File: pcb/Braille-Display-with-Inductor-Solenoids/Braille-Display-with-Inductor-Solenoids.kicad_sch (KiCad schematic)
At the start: 30 parts, among them J1 Screw_Terminal_01x02, J2 Screw_Terminal_01x02, J4 Conn_01x03, J5 Conn_01x02, J6 Conn_01x08, J7 Screw_Terminal_01x02, J8 Barrel_Jack_Switch, U1 RP2040-Zero, U103 INA219AxD

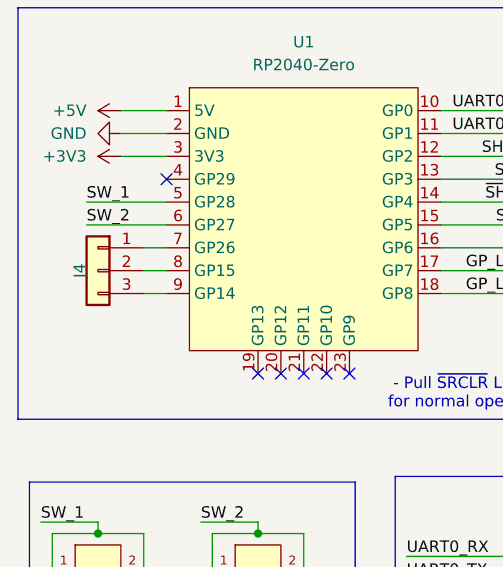
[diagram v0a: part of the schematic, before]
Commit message: pcb: WIP - High power and repeated routing
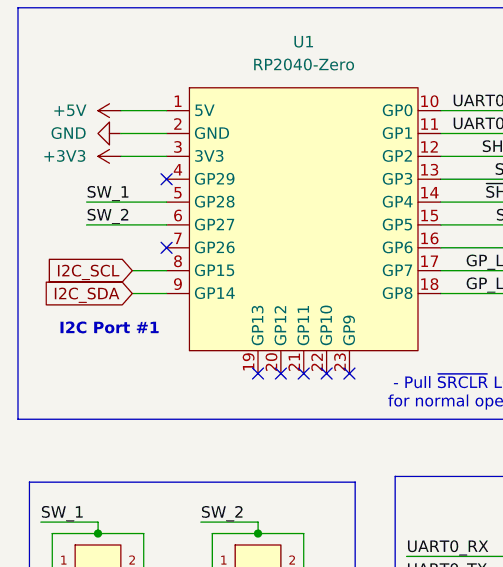
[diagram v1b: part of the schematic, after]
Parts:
- removed J4: Conn_01x03, Connector_PinHeader_2.54mm:PinHeader_1x03_P2.54mm_Vertical, symbol Connector_Generic:Conn_01x03
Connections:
- net I2C_SCL: now also U1.8 (GP15)
- net I2C_SDA: now also U1.9 (GP14)
- no-connect marks 17 -> 18
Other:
- note added: "I2C Port #1"
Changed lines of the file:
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@@
 		)
 	)
+	(text "I2C Port #1"
+		(exclude_from_sim no)
+		(at 24.13 49.784 0)
+		(effects
+			(font
+				(size 1.27 1.27)
+				(thickness 0.254)
+				(bold yes)
+			)
+		)
+	)
 	(text "SOICbite"
 		(exclude_from_sim no)
@@
 	)
 	(no_connect
+		(at 30.48 40.64)
+	)
+	(no_connect
 		(at 48.26 54.61)
 	)
@@
 	(wire
 		(pts
+			(xy 26.67 45.72) (xy 30.48 45.72)
+		)
+		(stroke
+			(width 0)
+			(type default)
+		)
+	)
+	(wire
+		(pts
 			(xy 17.78 76.2) (xy 17.78 72.39)
 		)
@@
 	(wire
 		(pts
+			(xy 26.67 43.18) (xy 30.48 43.18)
+		)
+		(stroke
+			(width 0)
+			(type default)
+		)
+	)
+	(wire
+		(pts
 			(xy 228.6 22.86) (xy 228.6 25.4)
 		)
@@
 	(wire
 		(pts
-			(xy 27.94 45.72) (xy 30.48 45.72)
-		)
-		(stroke
-			(width 0)
-			(type default)
-		)
-	)
-	(wire
-		(pts
 			(xy 228.6 52.07) (xy 228.6 50.8)
 		)
@@
 	(wire
 		(pts
-			(xy 27.94 43.18) (xy 30.48 43.18)
-		)
-		(stroke
-			(width 0)
-			(type default)
-		)
-	)
-	(wire
-		(pts
 			(xy 60.96 33.02) (xy 86.36 33.02)
 		)
@@
 	(wire
 		(pts
-			(xy 27.94 40.64) (xy 30.48 40.64)
-		)
-		(stroke
-			(width 0)
-			(type default)
-		)
-	)
-	(wire
-		(pts
 			(xy 78.74 182.88) (xy 78.74 179.07)
 		)
@@
 		)
 	)
+	(global_label "I2C_SDA"
+		(shape input)
+		(at 26.67 45.72 180)
+		(fields_autoplaced yes)
+		(effects
+			(font
+				(size 1.27 1.27)
+			)
+			(justify right)
+		)
+		(property "Intersheetrefs" "${INTERSHEET_REFS}"
+			(at 16.1253 45.72 0)
+			(effects
+				(font
+					(size 1.27 1.27)
+				)
+				(justify right)
+				(hide yes)
+			)
+		)
+	)
 	(global_label "I2C_SCL"
 		(shape input)
@@
 	(global_label "I2C_SCL"
 		(shape input)
+		(at 26.67 43.18 180)
+		(fields_autoplaced yes)
+		(effects
+			(font
+				(size 1.27 1.27)
+			)
+			(justify right)
+		)
+		(property "Intersheetrefs" "${INTERSHEET_REFS}"
+			(at 16.0648 43.18 0)
+			(effects
+				(font
+					(size 1.27 1.27)
+				)
+				(justify right)
+				(hide yes)
+			)
+		)
+	)
+	(global_label "I2C_SCL"
+		(shape input)
 		(at 135.89 196.85 0)
 		(fields_autoplaced yes)
@@
 					(unit 1)
 				)
-			)
-		)
-	)
-	(symbol
-		(lib_id "Connector_Generic:Conn_01x03")
-		(at 22.86 43.18 0)
-		(mirror y)
-		(unit 1)
-		(exclude_from_sim no)
-		(in_bom yes)
-		(on_board yes)
-		(dnp no)
-		(property "Reference" "J4"
-			(at 20.828 43.18 90)
-			(effects
-				(font
-					(size 1.27 1.27)
-				)
-			)
-		)
-		(property "Value" "Conn_01x03"
-			(at 22.86 36.83 0)
-			(effects
-				(font
-					(size 1.27 1.27)
-				)
-				(hide yes)
-			)
-		)
-		(property "Footprint" "Connector_PinHeader_2.54mm:PinHeader_1x03_P2.54mm_Vertical"
-			(at 22.86 43.18 0)
-			(effects
-				(font
-					(size 1.27 1.27)
-				)
-				(hide yes)
-			)
-		)
-		(property "Datasheet" "~"
-			(at 22.86 43.18 0)
-			(effects
-				(font
-					(size 1.27 1.27)
-				)
-				(hide yes)
-			)
-		)
-		(property "Description" "Generic connector, single row, 01x03, script generated (kicad-library-utils/schlib/autogen/connector/)"
-			(at 22.86 43.18 0)
-			(effects
-				(font
-					(size 1.27 1.27)
-				)
-				(hide yes)
-			)
-		)
-		(pin "3"
-		)
-		(pin "2"
-		)
-		(pin "1"
-		)
-		(instances
-			(project ""
-				(path "/3829a125-89bd-48f9-bfbe-92d753eb8f7f"
-					(reference "J4")
-					(unit 1)
-				)
